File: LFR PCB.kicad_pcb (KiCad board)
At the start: 2 copper layers, 91.3 x 173 mm, 60 parts, among them J1 BLUETOOTH, J10 jumper, J11 jumper, J12 jumper, J13 jumper, J14 jumper, J15 jumper, J16 jumper, J2 RLS08, J3 MOTOR 1, J4 MOTOR 2, J5 POWER IN, J6 I2C HEADER, J8 jumper, J9 jumper, SW1 Start, U1 ROB-14450, U2 LM7805_TO220

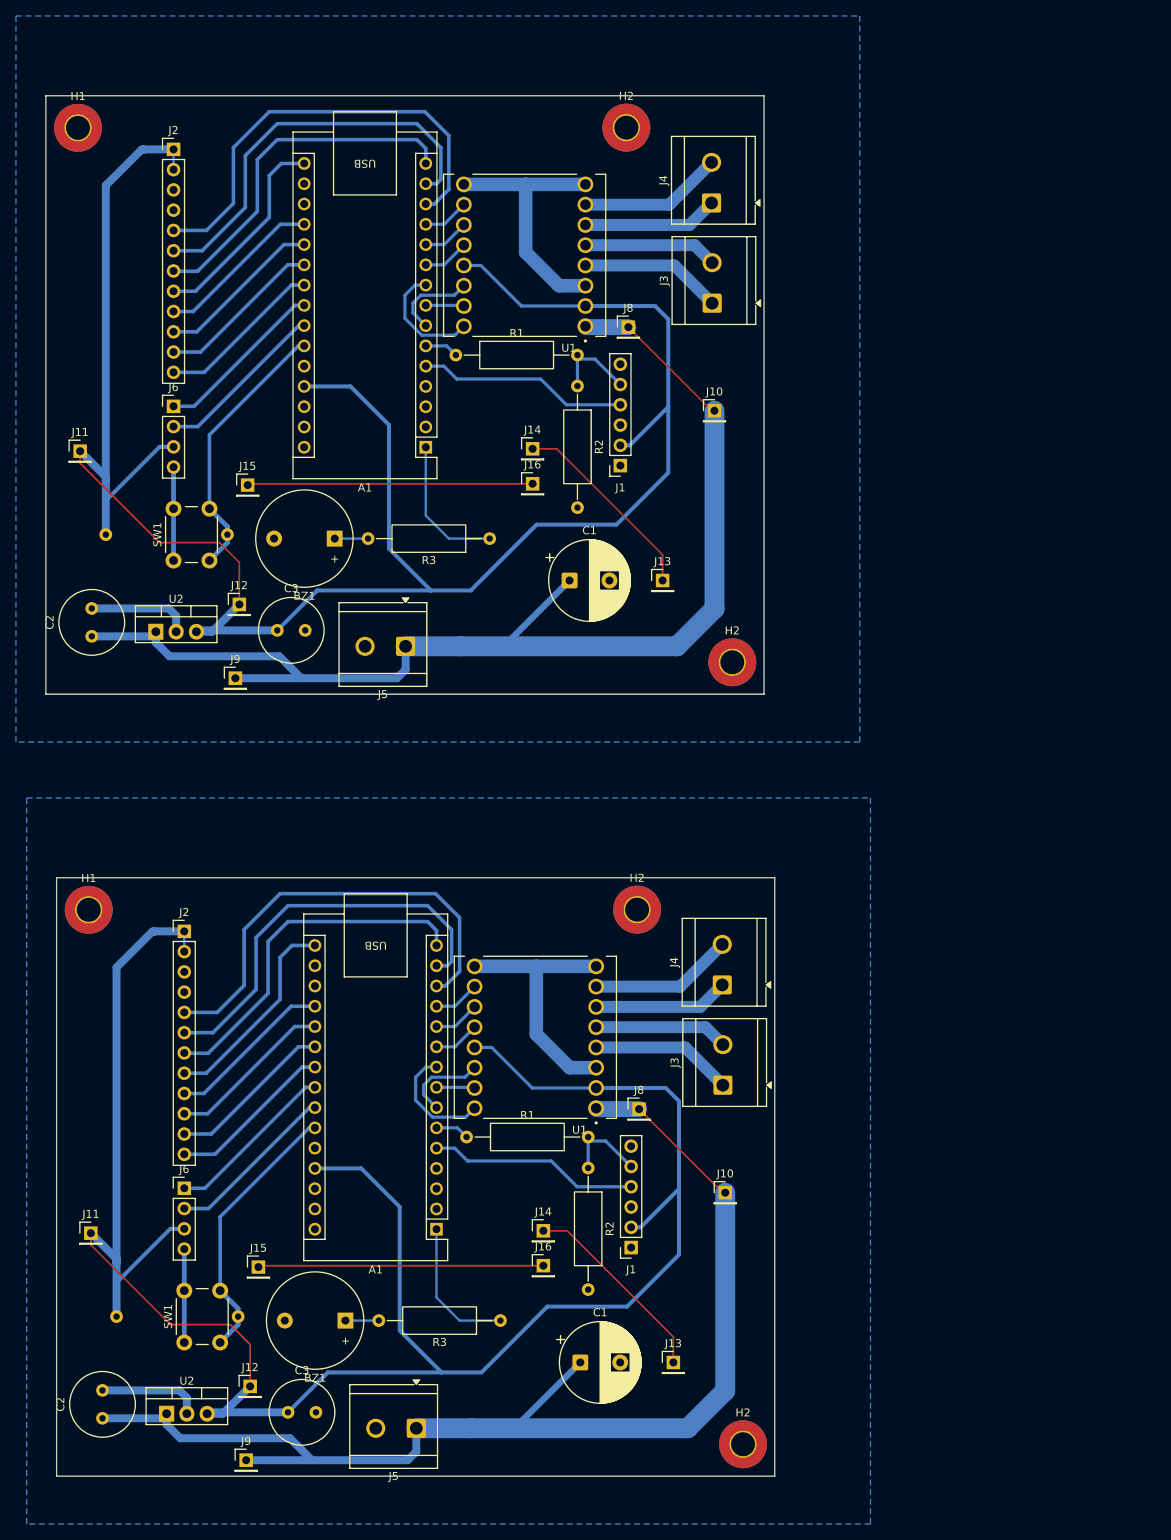
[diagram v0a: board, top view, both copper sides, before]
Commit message: Code
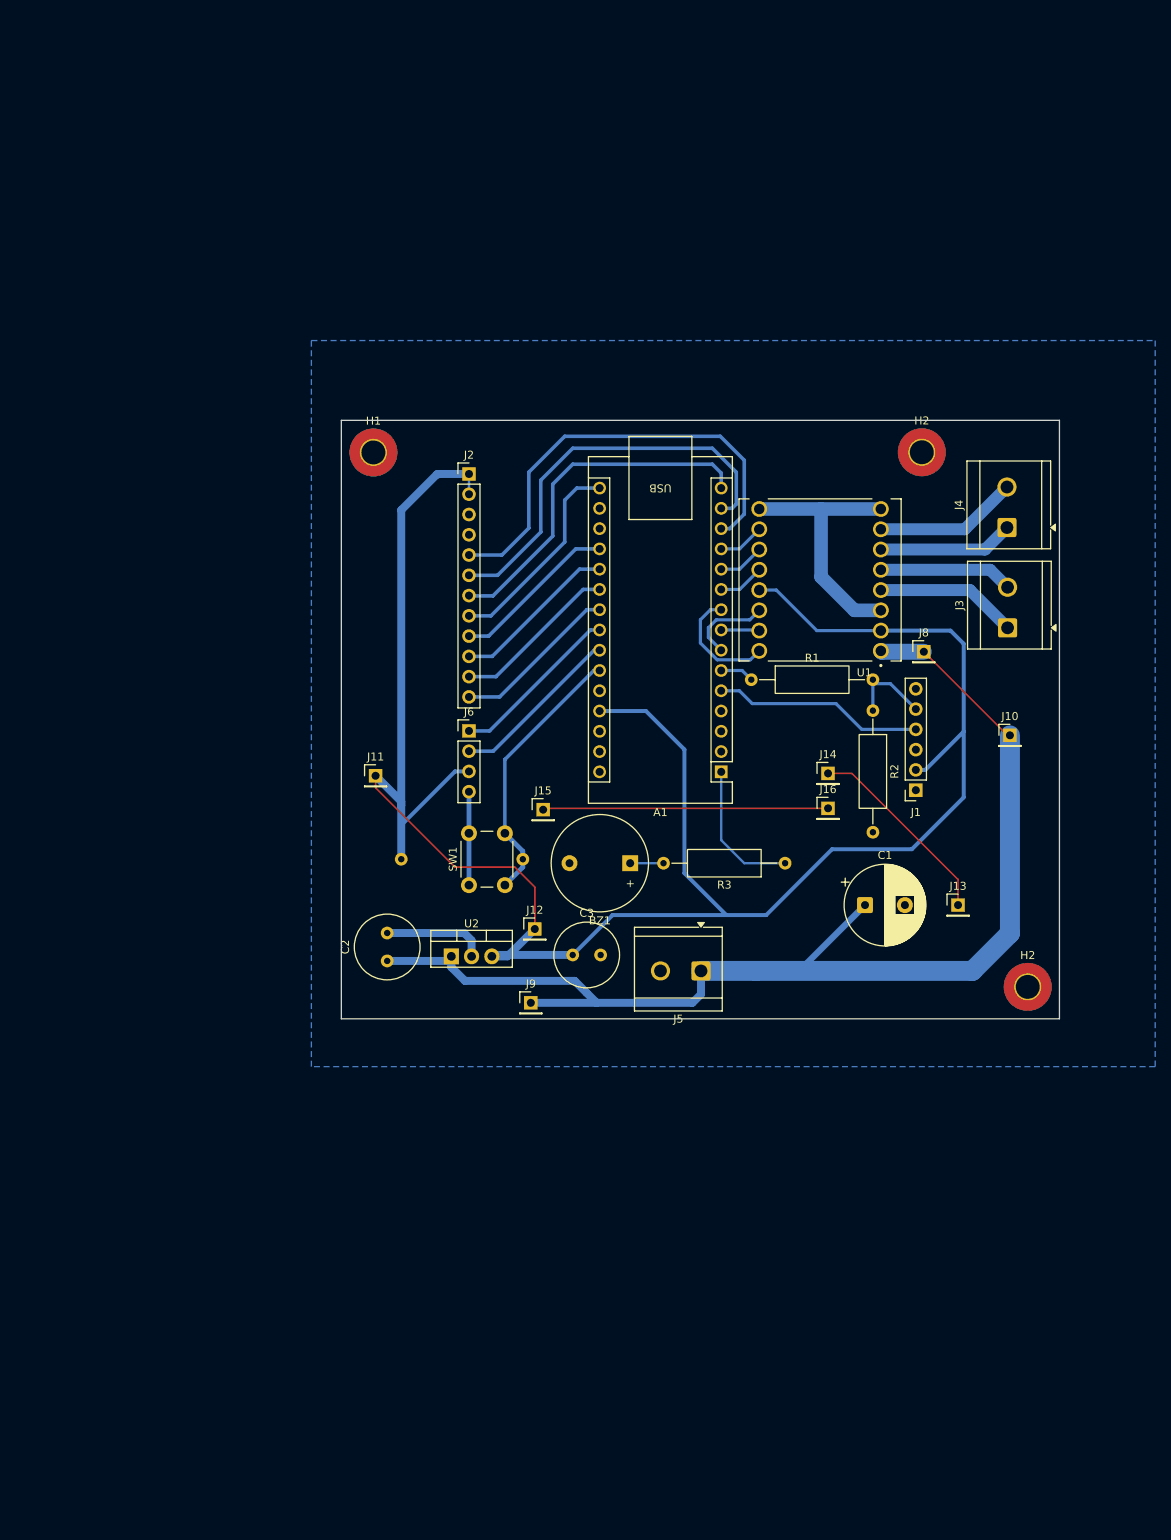
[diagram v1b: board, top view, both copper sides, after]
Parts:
- removed the A1 at (122.9, 158.1)
- removed the BZ1 at (111.5, 169.6)
- removed the C1 at (141.0, 174.8)
- removed the C2 at (81.1, 181.8)
- removed the C3 at (104.3, 181.1)
- removed the H1 at (79.3, 118.1)
- removed the H2 at (161.3, 185.1)
- removed the H2 at (148.1, 118.1)
- removed the J1 at (147.3, 160.4)
- removed the J10 at (159.1, 153.5)
- removed the J11 at (79.6, 158.6)
- removed the J12 at (99.6, 177.8)
- removed the J13 at (152.6, 174.8)
- removed the J14 at (136.3, 158.3)
- removed the J15 at (100.6, 162.9)
- removed the J16 at (136.3, 162.7)
- removed the J2 at (91.3, 120.8)
- removed the J3 at (158.8, 140.1)
- removed the J4 at (158.7, 127.5)
- removed the J5 at (120.4, 183.1)
- removed the J6 at (91.3, 153.0)
- removed the J8 at (148.3, 143.1)
- removed the J9 at (99.1, 187.1)
- removed the R1 at (126.7, 146.6)
- removed the R2 at (141.9, 150.4)
- removed the R3 at (130.9, 169.6)
- removed the R4 at (82.8, 169.1)
- removed the SW1 at (91.3, 172.3)
- removed the U1 at (135.3, 134.1)
- removed the U2 at (89.1, 181.2)
- moved A1 55.0 mm to (158.6, 100.8)
- moved C1 55.0 mm to (176.6, 117.5)
- moved C2 55.0 mm to (116.8, 124.5)
- moved C3 55.0 mm to (140.0, 123.8)
- moved H1 55.0 mm to (115.0, 60.8)
- moved H2 55.0 mm to (197.0, 127.8)
- moved H2 55.0 mm to (183.8, 60.8)
- moved J11 55.0 mm to (115.3, 101.3)
- moved J12 55.0 mm to (135.2, 120.5)
- moved J14 55.0 mm to (172.0, 101.0)
- moved J16 55.0 mm to (172.0, 105.4)
- moved J2 55.0 mm to (127.0, 63.5)
- moved J3 55.0 mm to (194.5, 82.8)
- moved J4 55.0 mm to (194.4, 70.2)
- moved J5 55.0 mm to (156.1, 125.8)
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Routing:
- net +5V: track 549.0 -> 274.5 mm
- net VBUS: track 315.0 -> 157.5 mm
- net GND: track 236.9 -> 118.4 mm
- net /D1: track 112.8 -> 56.4 mm
- net /D2: track 102.5 -> 51.3 mm
- net /D3: track 89.2 -> 44.6 mm
- net Net-(A1-A6): track 68.2 -> 34.1 mm
- net /TXD: track 52.8 -> 26.4 mm
- net /D4: track 52.2 -> 26.1 mm
- net /SCL: track 43.2 -> 21.6 mm
- net /SDA: track 43.2 -> 21.6 mm
- net /D6: track 41.8 -> 20.9 mm
- net /D7: track 41.8 -> 20.9 mm
- net /D5: track 41.8 -> 20.9 mm
- net /D8: track 41.8 -> 20.9 mm
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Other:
- board size 91.3 x 173 mm -> 90 x 75 mm
